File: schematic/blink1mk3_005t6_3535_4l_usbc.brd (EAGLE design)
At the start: 18.9 x 10.4 mm, 19 parts, among them J1 DX07P024AJ1R1500, T0A TPTP15R, T1B TPTP15R, U1 EFM32HG309F64G

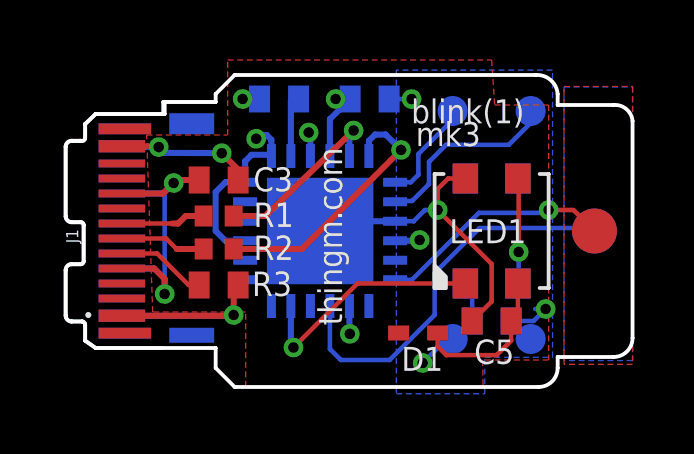
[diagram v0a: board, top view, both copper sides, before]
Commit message: more usbc work
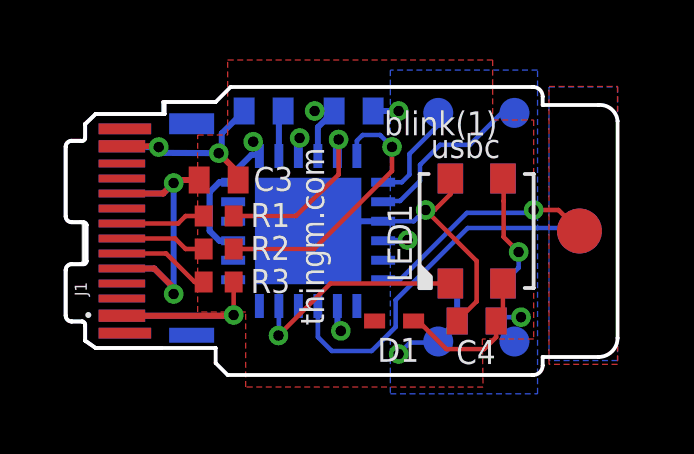
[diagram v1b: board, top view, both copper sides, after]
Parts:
- removed +5: TPTP10R, testpad:TP10R
- added 5V: TPTP10R, testpad:TP10R
- C1, C2, C4, C5: device adafruit:C0402 -> rcl:C0402
- C3: value 4.7uF -> 1uF; device adafruit:C0402 -> rcl:C0402
- LED1: value SK6812MINI -> WS2812B3535; device adafruit:LED3535 -> todstuff:LED3535
- R3: device adafruit:R0402 -> rcl:R0402
- moved D1 0.89 mm to (6.20, -3.00)
- moved C2 0.67 mm to (4.80, 4.00)
- moved C1 0.65 mm to (1.80, 4.00)
- moved G 0.55 mm to (10.2, -3.68)
- moved D 0.54 mm to (10.2, 3.94)
- moved C4 0.50 mm to (8.90, -3.00), flipped to the top
- moved C5 0.50 mm to (8.90, -3.00), flipped to the bottom
- moved LED1 0.50 mm to (8.90, 0.00)
- moved LED2 0.50 mm to (8.90, 0.00)
- moved T0A 0.50 mm to (12.3, 0.00)
- moved T1B 0.50 mm to (12.3, 0.00)
- moved C 0.48 mm to (7.62, 3.94)
- moved U1 0.40 mm to (3.28, 0.00)
- moved R3 0.10 mm to (0.30, -1.70)
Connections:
- net +5V: now also 5V.TP, C5.1; no longer +5.TP, C4.1
- net VLEDA: now also C4.1; no longer C5.1
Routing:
- net +3V3: track 10.8 -> 9.22 mm
- net CAP0A: track 13.1 -> 12.2 mm
- net DI: track 8.03 -> 7.45 mm
- net DECOUPLE: track 2.13 -> 1.56 mm
- net DBG_SWDIO: track 6.44 -> 5.92 mm
- net GND: track 29.1 -> 29.2 mm, vias 7 -> 6
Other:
- board size 18.9 x 10.4 mm -> 18.4 x 9.6 mm
- board text added: "354lc"
- board text added: "usbc"
- board text removed: "504l"
- board text removed: "mk3"
